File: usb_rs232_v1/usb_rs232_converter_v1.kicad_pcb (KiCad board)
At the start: 2 copper layers, 85 x 51 mm, 58 parts, among them CON1 USB-micro-B, CON2 USB-mini-B, IC1 MAX3243, IC2 FT232BL, J1 COM LEFT, J2 COM RIGHT, J3 FTDI, J4 COM RIGHT FTDI, J5 UART, J6 COM LEFT COM, J7 COM RIGHT COM

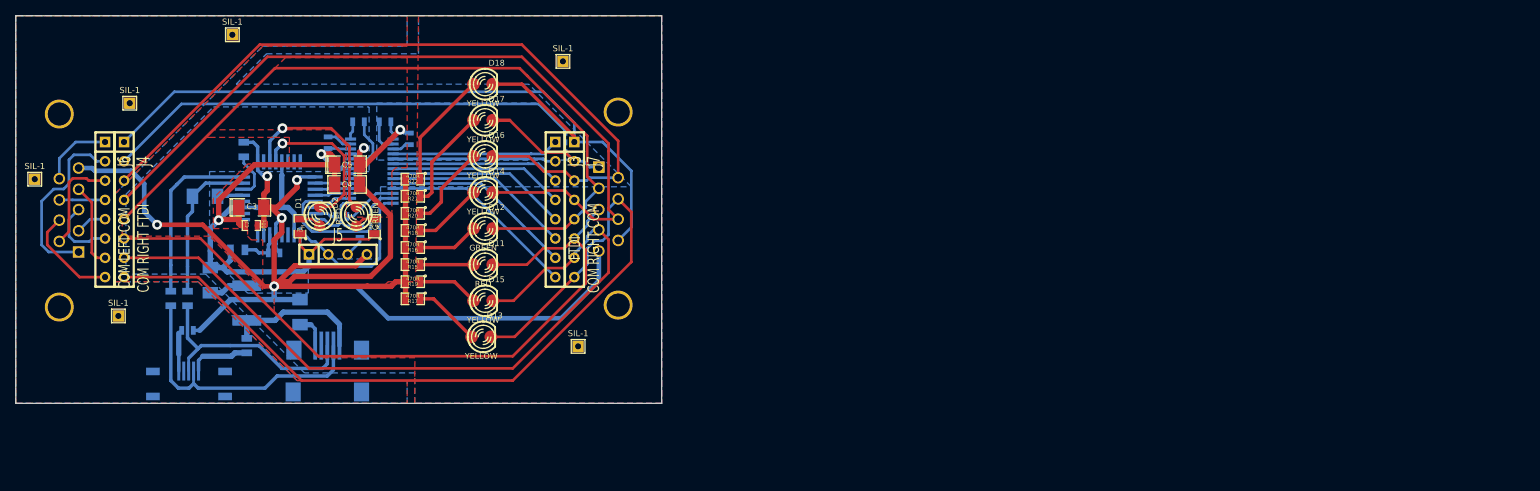
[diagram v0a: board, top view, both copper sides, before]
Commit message: usb_rs232 pcb_v2.0
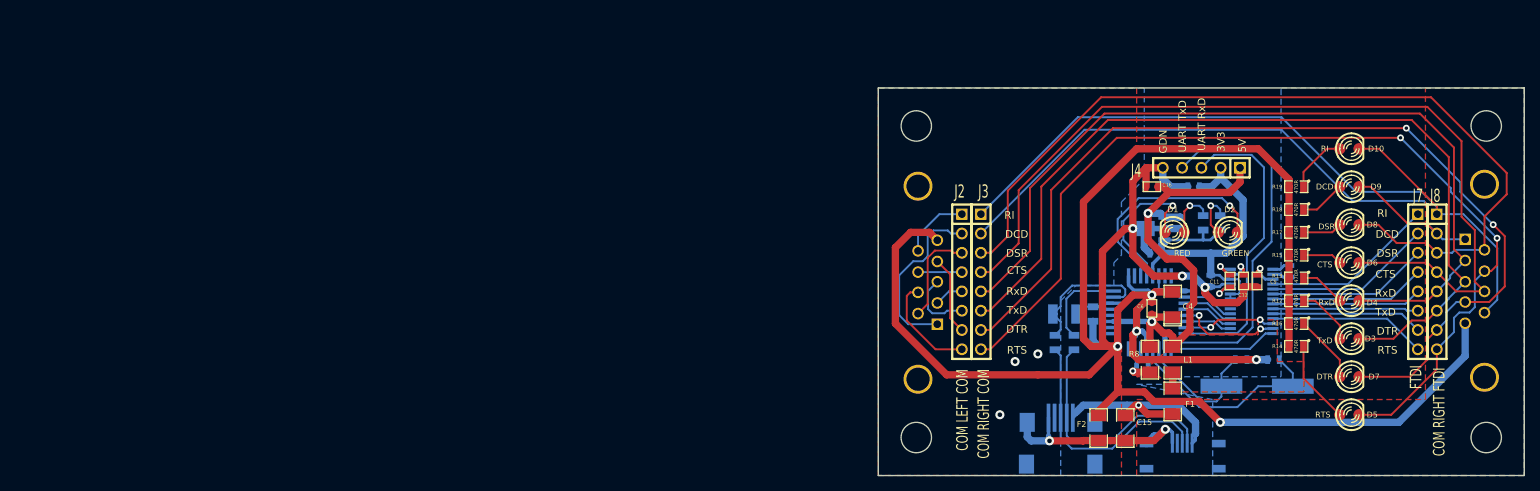
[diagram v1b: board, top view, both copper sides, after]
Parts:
- removed D11: RED, LED-3MM-SMD
- removed D12: GREEN, LED-3MM-SMD
- removed D13, D14, D15, D16, D17, D18: YELLOW, LED-3MM-SMD
- removed J5: UART, SIL-4
- removed R1, R20, R21, R22: 470R, SM0805
- removed R2, R3: 27R, SM0805
- removed R4: 1k5, SM1206
- removed R9: 0R, SM1206
- removed SIL-1 (x6): Val**, SIL-1
- added C1: 27p, SM0603, B.Cu at (183.8, 64.8)
- added C13: 100n, SM0603, B.Cu at (177.5, 42.0)
- added C14: 100n, SM0603, B.Cu at (175.8, 46.8)
- added C15: 4n7, SM1206, F.Cu at (168.5, 73.8)
- added C16: 100n, SM0603, F.Cu at (172.0, 42.0)
- added C6: 100n, SM0603, F.Cu at (172.0, 58.0)
- added D10: RI, LED-3MM-SMD, F.Cu at (198.0, 37.0)
- added D3: TxD, LED-3MM-SMD, F.Cu at (198.0, 62.0)
- added D4: RxD, LED-3MM-SMD, F.Cu at (198.0, 57.0)
- added D5: RTS, LED-3MM-SMD, F.Cu at (198.0, 72.0)
- added D6: CTS, LED-3MM-SMD, F.Cu at (198.0, 52.0)
- added D7: DTR, LED-3MM-SMD, F.Cu at (198.0, 67.0)
- added D8: DSR, LED-3MM-SMD, F.Cu at (198.0, 47.0)
- added D9: DCD, LED-3MM-SMD, F.Cu at (198.0, 42.0)
- added F2: 500mA, SM1206, F.Cu at (165.0, 73.8)
- added J8: COM RIGHT FTDI, SIL-8_bigger_hole, F.Cu at (209.5, 54.5)
- added R12: 470R, SM0805, F.Cu at (191.0, 57.0)
- added R13: 470R, SM0805, F.Cu at (191.0, 54.0)
- added R14: 470R, SM0805, F.Cu at (191.0, 63.0)
- added VR1: MC78L33, sot89, B.Cu at (171.8, 47.5)
- added X1: QUARTZCMS4_M, Q_49U3HMS, B.Cu at (185.8, 68.2)
- C10, C7, C8: value C -> 100n; footprint SM0603_Capa -> SM0603
- C11: value C -> 100n; footprint SM0603_Capa -> SM0603; moved to F.Cu
- C12: value 33n -> 100n; footprint SM0805 -> SM0603; moved to F.Cu
- C2: value 100n -> 33n; footprint SM0603_Capa -> SM0805; moved to B.Cu
- C3: value 10u -> 27p; footprint SM1206POL -> SM0603; moved to B.Cu
- C4: value 100n -> 10u; footprint SM1206 -> SM1206POL
- C5: value 10u -> 100n; footprint SM1206POL -> SM0603; moved to B.Cu
- C9: footprint SM0603_Capa -> SM0603; moved to F.Cu
- F1: value FUSE -> 500mA; footprint SM1812 -> SM1206; moved to F.Cu
- IC1: value MAX3243 -> FT232BL; footprint tssop-28 -> TQFP32
- IC2: value FT232BL -> MAX3243; footprint TQFP32 -> tssop-28
- J2: value COM RIGHT -> COM LEFT COM; footprint DB9MC-v2 -> SIL-8_bigger_hole; moved to F.Cu
- J3: value FTDI -> COM RIGHT COM; footprint SIL-8 -> SIL-8_bigger_hole
- J4: value COM RIGHT FTDI -> UART; footprint SIL-8 -> SIL-5_bigger_holes
- J6: value COM LEFT COM -> COM RIGHT; footprint SIL-8 -> DB9MC-v2; moved to B.Cu
- J7: value COM RIGHT COM -> FTDI; footprint SIL-8 -> SIL-8_bigger_hole
- L1: value INDUCTOR_SMALL -> 15uH; moved to F.Cu
- R10, R11: value 0R -> 470R; footprint SM0603 -> SM0805
- R5, R6: value R -> 27R; moved to B.Cu
- R7: value 0R -> 1k5; footprint SM0603 -> SM1210
- R8: value 0R -> 470R; footprint SM0805 -> SM1206; moved to F.Cu
- moved J6 180.5 mm to (214.5, 54.5), turned to 90 degrees
- moved J4 140.6 mm to (177.2, 39.5), turned to 180 degrees
- moved C3 136.0 mm to (188.0, 64.8), turned to 180 degrees
- moved R10 134.4 mm to (178.8, 46.8), turned to 90 degrees
- moved C12 132.7 mm to (184.1, 54.4)
- moved CON1 131.1 mm to (176.0, 79.0)
- moved C9 129.4 mm to (185.8, 54.4), turned to 90 degrees
- moved IC2 128.7 mm to (185.1, 57.1), turned to 270 degrees
- moved L1 127.1 mm to (174.8, 64.8)
- moved C8 124.1 mm to (190.2, 53.1), turned to 90 degrees
- moved F1 122.5 mm to (174.8, 70.2)
- moved C11 120.1 mm to (182.3, 54.4)
- moved R8 118.9 mm to (171.8, 64.8)
- moved R19 116.9 mm to (191.0, 42.0)
- moved R16 116.7 mm to (191.0, 60.0)
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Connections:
- C10 pad 1: GND -> +3.3V
- C10 pad 2: N-0000034 -> GND
- C11 pad 1: N-000006 (its old number) -> N-000001
- C11 pad 2: VCC -> N-000005
- C12 pad 1: GND -> N-0000010
- C12 pad 2: N-000001 -> GND
- C2 pad 2: VCC -> N-0000034
- C3 pad 1: VCC -> /XTOUT
- C4 pad 1: VCC -> +5V
- C5 pad 1: VCC -> GND
- C5 pad 2: GND -> /AVCC
- C7 pad 1: N-000004 -> GND
- C7 pad 2: N-000005 -> +3.3V
- C8 pad 1: N-0000033 -> N-000008
- C8 pad 2: N-0000032 -> N-000009
- C9 pad 2: N-0000055 -> N-000007
- CON1 pad 1: N-000008 -> N-0000057
- CON1 pad 5: N-0000052 -> N-0000039
- CON1 pad 8: GND -> N-0000039
- CON2 pad 1: /USB Vcc -> N-0000057
- CON2 pad 6: (no net) -> N-0000039
- CON2 pad 9: GND -> (no net)
- D1 pad 1: N-0000026 -> N-0000012
- D2 pad 1: N-0000025 -> N-0000011
- F1 pad 1: /USB Vcc -> N-0000057
- IC1 pad 1: N-000005 -> (no net)
- IC1 pad 10: /Tout: DTR -> (no net)
- IC1 pad 11: /Tout: RST -> /RX LED
- IC1 pad 12: /Tin: RST2 -> /TX LED
- IC1 pad 13: /Tin: DTR -> +3.3V
- IC1 pad 14: /Tin: TxD -> GND
- IC1 pad 15: /Rout: RxD -> (no net)
- IC1 pad 16: /Rout: CTS -> (no net)
- IC1 pad 17: /Rout: DSR -> GND
- IC1 pad 18: /Rout: DCD -> /Rout: RI
- IC1 pad 19: /Rout: RI -> /Rout: DCD
- IC1 pad 2: N-000004 -> (no net)
- IC1 pad 20: (no net) -> /Rout: DSR
- IC1 pad 21: (no net) -> /Tin: DTR
- IC1 pad 22: VCC -> /Rout: CTS
- IC1 pad 23: VCC -> /Tin: RST
- IC1 pad 24: N-0000032 -> /Rout: RxD
- IC1 pad 25: GND -> /Tin: TxD
- IC1 pad 26: VCC -> +5V
- IC1 pad 27: N-000006 (its old number) -> /XTIN
- IC1 pad 28: N-0000033 -> /XTOUT
- IC1 pad 3: N-0000034 -> +5V
- IC1 pad 4: /Rin: RI -> (no net)
- IC1 pad 5: /Rin: DCD -> (no net)
- IC1 pad 6: /Rin: DSR -> N-0000034
- IC1 pad 7: /Rin: CTS -> /D++
- IC1 pad 8: /Rin: RxD -> /D--
- IC1 pad 9: /Tout: TxD -> GND
- IC2 pad 1: (no net) -> N-000009
- IC2 pad 10: (no net) -> /Tout: DTR
- IC2 pad 11: /RX LED -> /Tout: RST
- IC2 pad 12: /TX LED -> /Tin: RST
- IC2 pad 13: VCC -> /Tin: DTR
- IC2 pad 14: (no net) -> /Tin: TxD
- IC2 pad 15: (no net) -> /Rout: RxD
- IC2 pad 16: (no net) -> /Rout: CTS
- IC2 pad 17: GND -> /Rout: DSR
- IC2 pad 18: /Rout: RI -> /Rout: DCD
- IC2 pad 19: /Rout: DCD -> /Rout: RI
- IC2 pad 2: (no net) -> N-000008
- IC2 pad 20: /Rout: DSR -> (no net)
- IC2 pad 21: /Tin: DTR -> (no net)
- IC2 pad 22: /Rout: CTS -> +3.3V
- IC2 pad 23: /Tin: RST -> +3.3V
- IC2 pad 24: /Rout: RxD -> N-000005
- IC2 pad 25: /Tin: TxD -> GND
- IC2 pad 26: VCC -> +3.3V
- IC2 pad 27: (no net) -> N-0000010
- IC2 pad 28: (no net) -> N-000001
- IC2 pad 3: VCC -> N-000007
- IC2 pad 4: VCC -> /Rin: RI
- IC2 pad 5: N-000002 -> /Rin: DCD
- IC2 pad 6: N-000001 -> /Rin: DSR
- IC2 pad 7: /D++ -> /Rin: CTS
- IC2 pad 8: /D-- -> /Rin: RxD
- IC2 pad 9: GND -> /Tout: TxD
- J2 pad 1: /DCD COM -> /RI COM LEFT
- J2 pad 2: /RxD COM -> /DCD COM LEFT
- J2 pad 3: /TxD COM -> /DSR COM LEFT
- J2 pad 4: /DTR COM -> /CTS COM LEFT
- J2 pad 5: GND -> /RxD COM LEFT
- J2 pad 6: /DSR COM -> /TxD COM LEFT
- J2 pad 7: /RST COM -> /DTR COM LEFT
- J2 pad 8: /CTS COM -> /RST COM LEFT
- J3 pad 1: /Rin: RI -> /RI COM
- J3 pad 2: /Rin: DCD -> /DCD COM
- J3 pad 3: /Rin: DSR -> /DSR COM
- J3 pad 4: /Rin: CTS -> /CTS COM
- J3 pad 5: /Rin: RxD -> /RxD COM
- J3 pad 6: /Tout: TxD -> /TxD COM
- J3 pad 7: /Tout: DTR -> /DTR COM
- J3 pad 8: /Tout: RST -> /RST COM
- J4 pad 1: /RI COM -> +5V
- J4 pad 2: /DCD COM -> +3.3V
- J4 pad 3: /DSR COM -> /Rout: RxD
- J4 pad 4: /CTS COM -> /Tin: TxD
- J4 pad 5: /RxD COM -> GND
- J6 pad 1: /RI COM LEFT -> /DCD COM
- J6 pad 2: /DCD COM LEFT -> /RxD COM
- J6 pad 3: /DSR COM LEFT -> /TxD COM
- J6 pad 4: /CTS COM LEFT -> /DTR COM
- J6 pad 5: /RxD COM LEFT -> GND
- J6 pad 6: /TxD COM LEFT -> /DSR COM
- J6 pad 7: /DTR COM LEFT -> /RST COM
- J6 pad 8: /RST COM LEFT -> /CTS COM
- J7 pad 1: /RI COM -> /Rin: RI
- J7 pad 2: /DCD COM -> /Rin: DCD
- J7 pad 3: /DSR COM -> /Rin: DSR
- J7 pad 4: /CTS COM -> /Rin: CTS
- J7 pad 5: /RxD COM -> /Rin: RxD
- J7 pad 6: /TxD COM -> /Tout: TxD
- J7 pad 7: /DTR COM -> /Tout: DTR
- J7 pad 8: /RST COM -> /Tout: RST
- L1 pad 2: VCC -> +5V
- R10 pad 1: GND -> +3.3V
- R10 pad 2: N-0000052 -> N-0000012
- R11 pad 1: /Rout: RxD -> +3.3V
- R11 pad 2: N-0000053 -> N-0000011
- R5 pad 1: VCC -> /D-
- R5 pad 2: N-0000026 -> /D--
- R6 pad 1: VCC -> /D+
- R6 pad 2: N-0000025 -> /D++
- R7 pad 1: /Tin: RST2 -> N-0000034
- R7 pad 2: /Tin: RST -> /D++
- R8 pad 1: /USB Vcc -> +5V
- R8 pad 2: N-000008 -> /AVCC
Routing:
- net GND: track 234.6 -> 336.6 mm, vias 7 -> 11
- net VCC: track 99.9 -> 0.00 mm, vias 2 -> 0
- net +5V: track 0.00 -> 66.1 mm, vias 0 -> 2
- net +3.3V: track 0.00 -> 50.2 mm
- net /Tin: TxD: track 21.3 -> 62.7 mm
- net /Rout: RxD: track 10.2 -> 39.6 mm
- net N-0000057: track 0.00 -> 28.8 mm, vias 0 -> 1
- net /XTOUT: track 0.00 -> 27.9 mm
- net /DTR COM: track 99.7 -> 125.6 mm, vias 0 -> 2
- net N-0000039: track 4.43 -> 29.8 mm, vias 0 -> 2
- net /TxD COM: track 95.0 -> 114.0 mm
- net /USB Vcc: track 18.5 -> 0.00 mm
- net /XTIN: track 0.00 -> 17.8 mm
- net N-0000035: track 15.4 -> 0.00 mm
- net /DSR COM: track 100.6 -> 114.8 mm
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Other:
- outline, holes or cut-outs redrawn
- net class Default: trace_width 0.3556 -> 0.254; via_dia 1.3 -> 0.9; via_drill 0.9 -> 0.6
- net class power removed
- net class signal added: clearance 0.2032, trace_width 0.254, via_dia 0.9, via_drill 0.6
- net class small track removed
- net class supply added: clearance 0.2032, trace_width 0.7112, via_dia 1.2, via_drill 0.9
- rule via_min_drill: 0.9 -> 0.508
- rule via_min_size: 1.3 -> 0.889
- board text added: "3V3"
- board text added: "5V"
- board text added: "CTS"
- board text added: "DCD"
- board text added: "DSR"
- board text added: "DTR"
- board text added: "GDN"
- board text added: "RI"
- board text added: "RTS"
- board text added: "RxD"
- board text added: "TxD"
- board text added: "UART RxD"
- board text added: "UART TxD"
